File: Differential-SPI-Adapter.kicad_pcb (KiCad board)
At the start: 2 copper layers, 44.4 x 21.5 mm, 23 parts, among them J1 Conn_02x03_Odd_Even, J2 Conn_02x05_Odd_Even, J3 Conn_02x03_Odd_Even, J4 Conn_02x05_Odd_Even, U1 AM26LV31CD, U2 AM26LV32CD, U3 THVD1450D, U4 THVD1450D, U5 XC6206PxxxMR, U6 XC6206PxxxMR

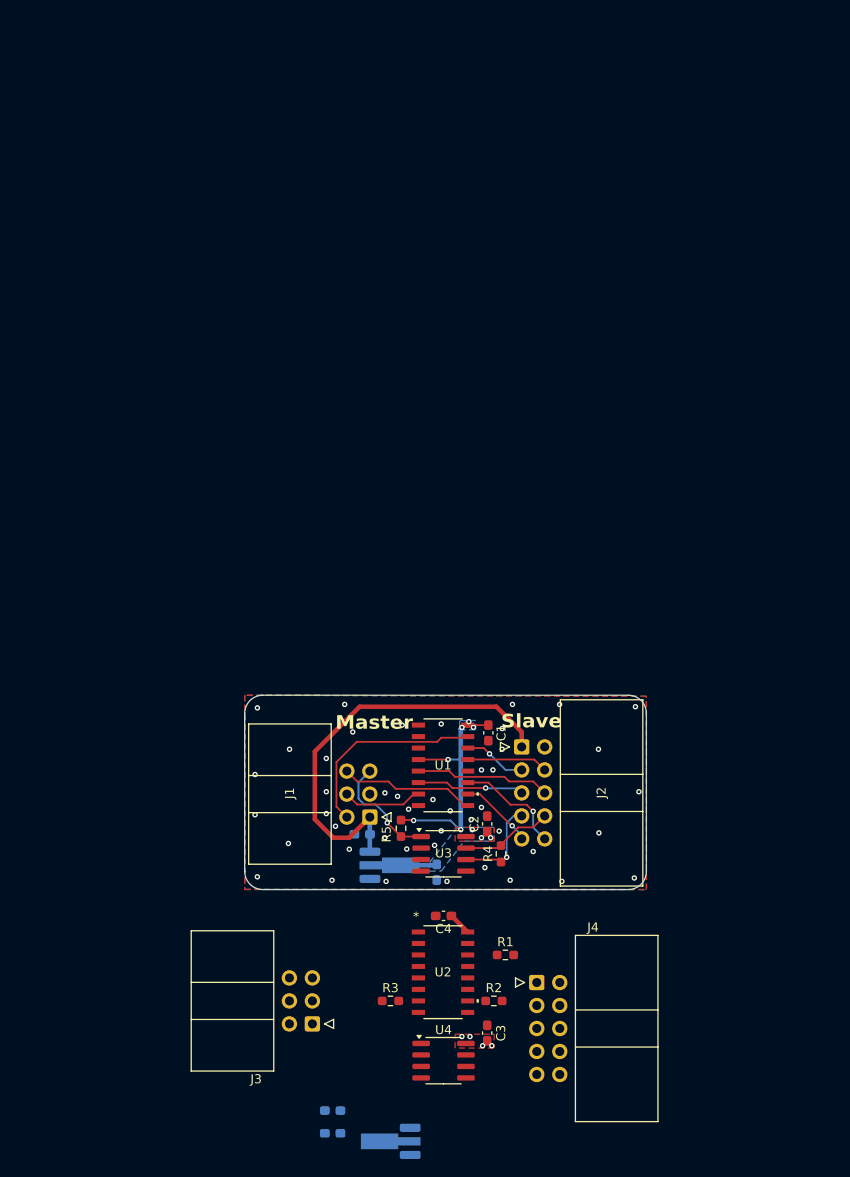
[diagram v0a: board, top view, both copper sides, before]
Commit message: reciever
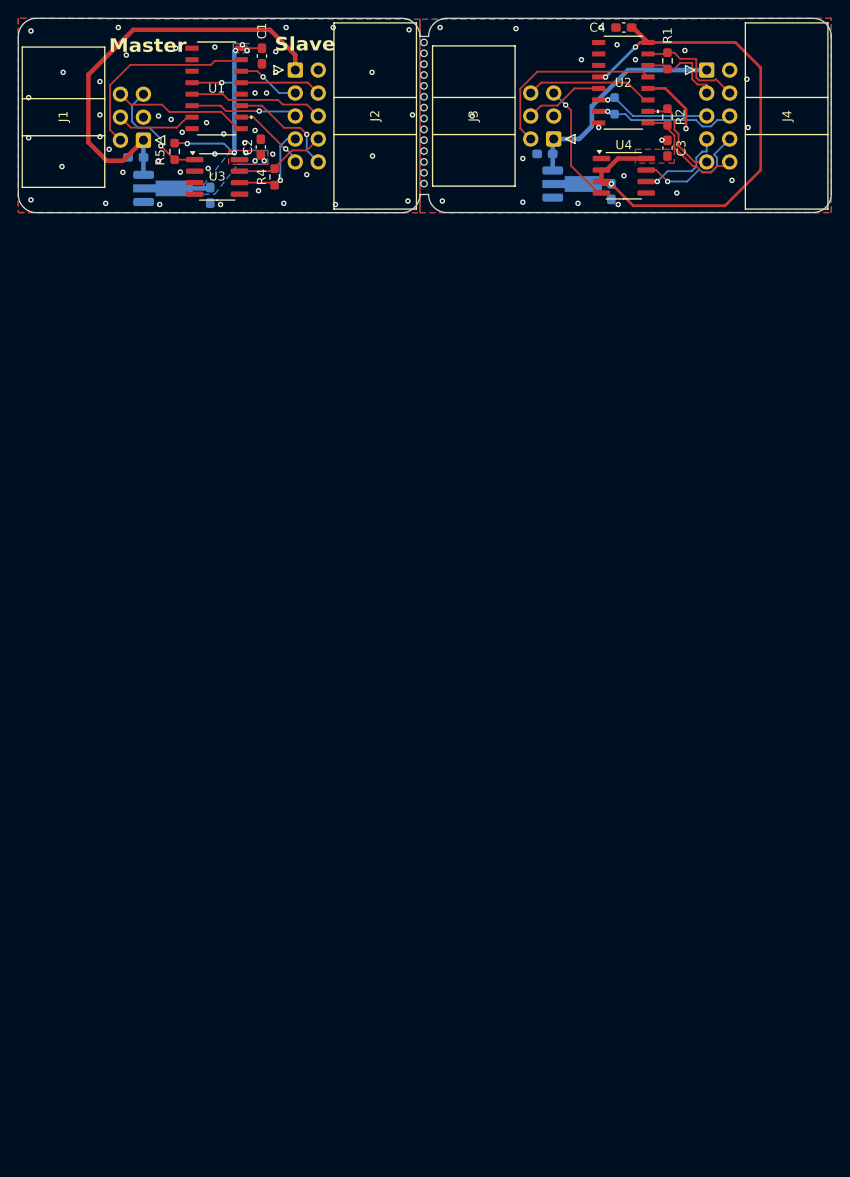
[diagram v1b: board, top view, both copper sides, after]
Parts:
- R3: moved to B.Cu
- moved C8 108.5 mm to (85.7, 38.8), turned to -90 degrees
- moved C7 108.3 mm to (78.4, 34.7)
- moved U6 107.8 mm to (81.7, 38.0), turned to 0 degrees
- moved J4 102.6 mm to (96.3, 25.4)
- moved R3 102.0 mm to (86.1, 29.4), turned to -90 degrees
- moved J3 101.4 mm to (79.4, 33.0)
- moved R1 100.4 mm to (91.9, 24.4), turned to -90 degrees
- moved U2 100.3 mm to (87.1, 26.8)
- moved C4 100.2 mm to (87.1, 20.7)
- moved C3 99.8 mm to (91.9, 34.0)
- moved U4 99.8 mm to (87.1, 37.1)
- moved R2 99.6 mm to (91.9, 30.6), turned to -90 degrees
- moved C5 78.9 mm to (33.2, 35.1)
- moved C6 78.9 mm to (41.4, 39.2)
- moved J2 78.9 mm to (50.8, 25.4)
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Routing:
- net +3.3VA: track 2.54 -> 68.7 mm, vias 4 -> 3
- net +5VA: track 0.00 -> 24.9 mm
- net /SCK_{2}: track 0.00 -> 21.2 mm
- net /MOSI_{2}-: track 0.00 -> 15.6 mm, vias 0 -> 1
- net /CS_{2}: track 0.00 -> 14.2 mm
- net /MISO_{2}: track 0.00 -> 13.4 mm, vias 0 -> 1
- net /MISO_{2}-: track 0.00 -> 13.2 mm, vias 0 -> 1
- net /MOSI_{2}+: track 0.00 -> 12.9 mm, vias 0 -> 1
- net /CS_{2}-: track 0.00 -> 12.9 mm
- net /SCK_{2}-: track 0.00 -> 12.2 mm
- net /CS_{2}+: track 0.00 -> 10.7 mm
- net /MISO_{2}+: track 0.00 -> 10.0 mm, vias 0 -> 1
- net /SCK_{2}+: track 0.00 -> 9.94 mm
- net /MOSI_{2}: track 0.00 -> 8.77 mm
- net GND: track 0.00 -> 8.45 mm, vias 45 -> 66
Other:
- board size 44.4 x 21.5 mm -> 89.8 x 21.5 mm
